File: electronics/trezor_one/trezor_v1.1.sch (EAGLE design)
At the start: 44 parts, among them IC1 MCP1703T-3302E/CB, K1 USB5_USB_MICRO_MOLEX475890001, K2 SWD, Q2 8MHz, U1 STM32F205RET6, U3 DISPLAY

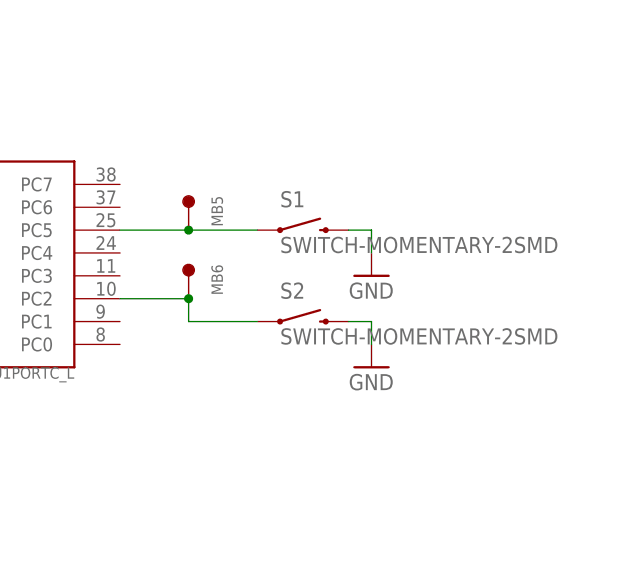
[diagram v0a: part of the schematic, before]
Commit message: Using 0603 passives, changed pushbutton
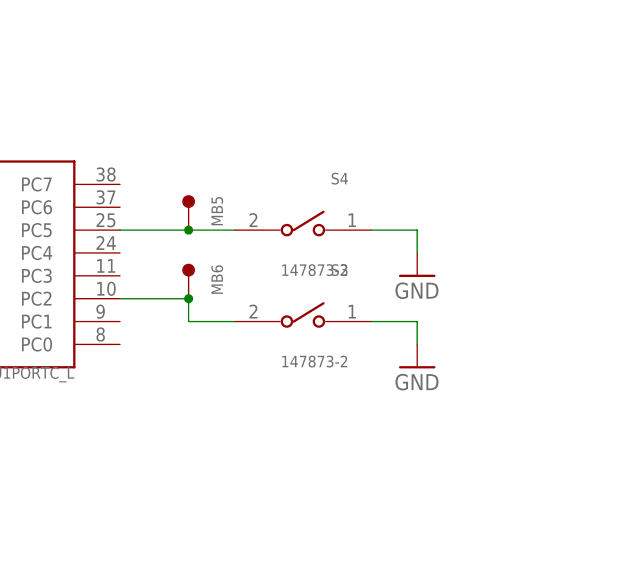
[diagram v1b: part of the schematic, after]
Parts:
- removed S1, S2: SWITCH-MOMENTARY-2SMD, SparkFun-Electromechanical:SWITCH-MOMENTARY-2SMD
- added S3, S4: 147873-2, 147873-2:147873-2
- C1, C12, C13, C14, C15, C16, C18, C2, C20, C21, C3, C4, C6, C7, C8, C9: device vyber:C_0402 -> vyber:C_0603
- R10, R3, R4, R6, R7, R8: device vyber:R_0402 -> vyber:R_0603
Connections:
- net GND: now also S3.1, S4.1; no longer S1.2, S2.2
- net N$19: now also S4.2; no longer S1.1
- net N$20: now also S3.2; no longer S2.1
